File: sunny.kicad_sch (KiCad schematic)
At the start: 53 parts, among them J2 Screw_Terminal_01x03, Q1 FQPF7N90C, T1 7508112339, U10 Optocoupler_DC_PhotoNPN_AKEC, U11 TL431D, U4 MIC4684, U5 UC3842N, U9 AP2112K-3.3, X2 B2P-VH

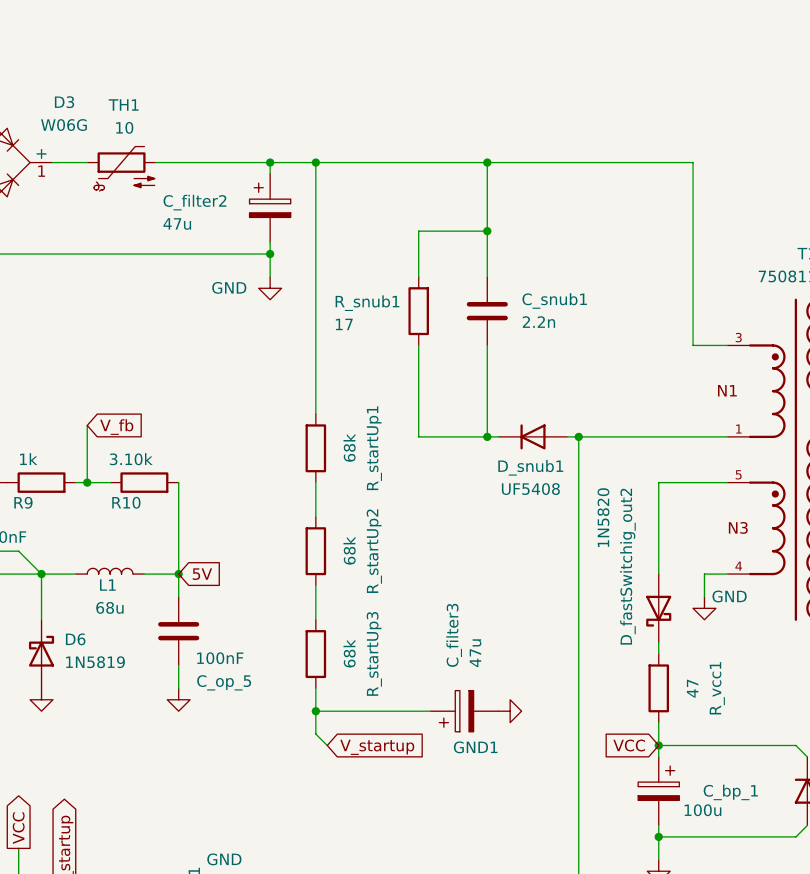
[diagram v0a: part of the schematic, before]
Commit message: Initialtes
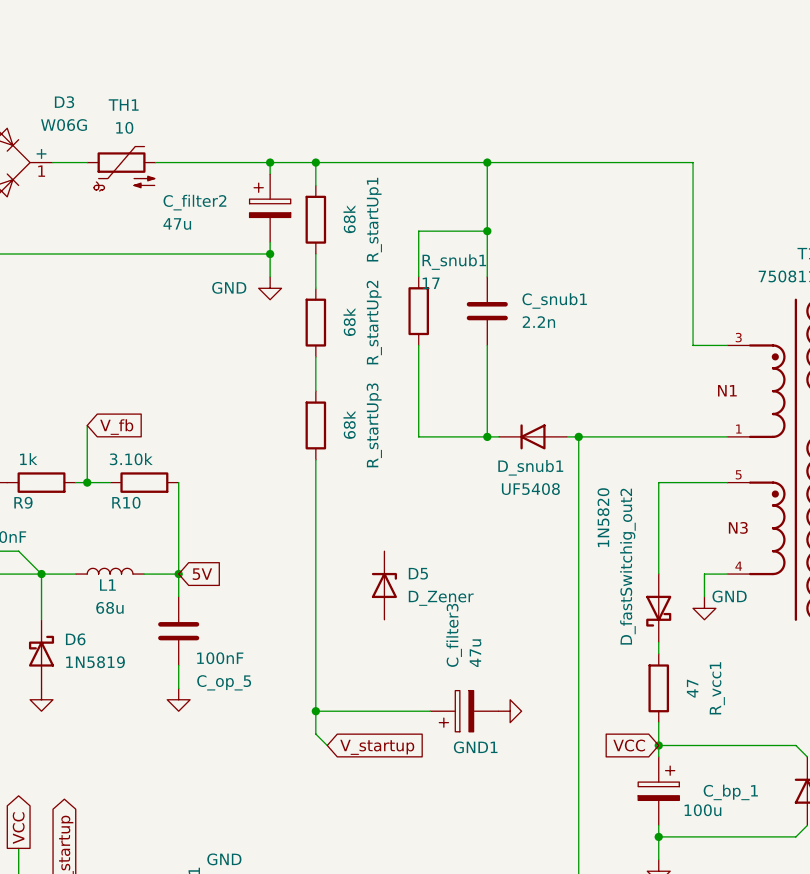
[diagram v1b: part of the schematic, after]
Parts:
- added D5: D_Zener, Diode_THT:D_5KP_P12.70mm_Horizontal, symbol Device:D_Zener
- U5: footprint UC3842N:DIP794W45P254L959H508Q8 -> kaam25_footprints_symbol:DIP794W45P254L959H508Q8
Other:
- moved on the sheet: R_startUp1, R_startUp2, R_startUp3
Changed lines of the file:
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@@
 	)
 	(junction
-		(at 148.59 38.1)
+		(at 186.69 102.87)
 		(diameter 0)
 		(color 0 0 0 0)
 	)
 	(junction
-		(at 186.69 102.87)
+		(at 76.2 81.28)
 		(diameter 0)
 		(color 0 0 0 0)
 	)
 	(junction
-		(at 76.2 81.28)
+		(at 148.59 99.06)
 		(diameter 0)
 		(color 0 0 0 0)
@@
 	)
 	(junction
-		(at 148.59 99.06)
+		(at 148.59 38.1)
 		(diameter 0)
 		(color 0 0 0 0)
@@
 	(wire
 		(pts
-			(xy 148.59 96.52) (xy 148.59 99.06)
+			(xy 148.59 71.12) (xy 148.59 99.06)
 		)
 		(stroke
@@
 	(wire
 		(pts
-			(xy 148.59 85.09) (xy 148.59 88.9)
+			(xy 148.59 59.69) (xy 148.59 63.5)
 		)
 		(stroke
@@
 	(wire
 		(pts
-			(xy 148.59 38.1) (xy 148.59 66.04)
+			(xy 148.59 38.1) (xy 148.59 40.64)
 		)
 		(stroke
@@
 	(wire
 		(pts
-			(xy 148.59 73.66) (xy 148.59 77.47)
+			(xy 148.59 48.26) (xy 148.59 52.07)
 		)
 		(stroke
@@
 			)
 		)
-		(property "Footprint" "UC3842N:DIP794W45P254L959H508Q8"
+		(property "Footprint" "kaam25_footprints_symbol:DIP794W45P254L959H508Q8"
 			(at 97.79 137.16 0)
 			(hide yes)
@@
 		(dnp no)
 		(property "Reference" "R_snub1"
-			(at 150.622 53.594 0)
+			(at 160.274 49.022 0)
 			(show_name no)
 			(do_not_autoplace no)
@@
 		)
 		(property "Value" "17"
-			(at 150.622 56.134 0)
+			(at 160.274 51.562 0)
 			(show_name no)
 			(do_not_autoplace no)
@@
 	(symbol
 		(lib_id "Device:R")
-		(at 148.59 92.71 0)
+		(at 148.59 67.31 0)
 		(mirror x)
 		(unit 1)
@@
 		(dnp no)
 		(property "Reference" "R_startUp3"
-			(at 154.94 92.71 90)
+			(at 154.94 67.31 90)
 			(show_name no)
 			(do_not_autoplace no)
@@
 		)
 		(property "Value" "68k"
-			(at 152.4 92.71 90)
+			(at 152.4 67.31 90)
 			(show_name no)
 			(do_not_autoplace no)
@@
 		)
 		(property "Footprint" "Resistor_THT:R_Axial_DIN0309_L9.0mm_D3.2mm_P20.32mm_Horizontal"
-			(at 146.812 92.71 90)
+			(at 146.812 67.31 90)
 			(hide yes)
 			(show_name no)
@@
 		)
 		(property "Datasheet" ""
-			(at 148.59 92.71 0)
+			(at 148.59 67.31 0)
 			(hide yes)
 			(show_name no)
@@
 		)
 		(property "Description" "starup voltage flows through before aux winding start supplying it, HV resistor, 0.5W, 310Volts"
-			(at 148.59 92.71 0)
+			(at 148.59 67.31 0)
 			(hide yes)
 			(show_name no)
@@
 	(symbol
 		(lib_id "Device:R")
-		(at 148.59 81.28 0)
+		(at 148.59 55.88 0)
 		(mirror x)
 		(unit 1)
@@
 		(dnp no)
 		(property "Reference" "R_startUp2"
-			(at 154.94 81.28 90)
+			(at 154.94 55.88 90)
 			(show_name no)
 			(do_not_autoplace no)
@@
 		)
 		(property "Value" "68k"
-			(at 152.4 81.28 90)
+			(at 152.4 55.88 90)
 			(show_name no)
 			(do_not_autoplace no)
@@
 		)
 		(property "Footprint" "Resistor_THT:R_Axial_DIN0309_L9.0mm_D3.2mm_P20.32mm_Horizontal"
-			(at 146.812 81.28 90)
+			(at 146.812 55.88 90)
 			(hide yes)
 			(show_name no)
@@
 		)
 		(property "Datasheet" ""
-			(at 148.59 81.28 0)
+			(at 148.59 55.88 0)
 			(hide yes)
 			(show_name no)
@@
 		)
 		(property "Description" "starup voltage flows through before aux winding start supplying it, HV resistor,0.5W, 310V"
-			(at 148.59 81.28 0)
+			(at 148.59 55.88 0)
 			(hide yes)
 			(show_name no)
@@
 	(symbol
 		(lib_id "Device:R")
-		(at 148.59 69.85 0)
+		(at 148.59 44.45 0)
 		(mirror x)
 		(unit 1)
@@
 		(dnp no)
 		(property "Reference" "R_startUp1"
-			(at 154.94 69.85 90)
+			(at 154.94 44.45 90)
 			(show_name no)
 			(do_not_autoplace no)
@@
 		)
 		(property "Value" "68k"
-			(at 152.4 69.85 90)
+			(at 152.4 44.45 90)
 			(show_name no)
 			(do_not_autoplace no)
@@
 		)
 		(property "Footprint" "Resistor_THT:R_Axial_DIN0309_L9.0mm_D3.2mm_P20.32mm_Horizontal"
-			(at 146.812 69.85 90)
+			(at 146.812 44.45 90)
 			(hide yes)
 			(show_name no)
@@
 		)
 		(property "Datasheet" ""
-			(at 148.59 69.85 0)
+			(at 148.59 44.45 0)
 			(hide yes)
 			(show_name no)
@@
 		)
 		(property "Description" "starup voltage flows through before aux winding start supplying it, HV resistor,0.5W, 310V"
-			(at 148.59 69.85 0)
+			(at 148.59 44.45 0)
 			(hide yes)
 			(show_name no)
@@
 					(unit 1)
 				)
+			)
+		)
+	)
+	(symbol
+		(lib_id "Device:D_Zener")
+		(at 156.21 85.09 270)
+		(unit 1)
+		(body_style 1)
+		(exclude_from_sim no)
+		(in_bom yes)
+		(on_board yes)
+		(in_pos_files yes)
+		(dnp no)
+		(fields_autoplaced yes)
+		(property "Reference" "D5"
+			(at 158.75 83.8199 90)
+			(show_name no)
+			(do_not_autoplace no)
+			(effects
+				(font
+					(size 1.27 1.27)
+				)
+				(justify left)
+			)
+		)
+		(property "Value" "D_Zener"
+			(at 158.75 86.3599 90)
+			(show_name no)
+			(do_not_autoplace no)
+			(effects
+				(font
+					(size 1.27 1.27)
+				)
+				(justify left)
+			)
+		)
+		(property "Footprint" "Diode_THT:D_5KP_P12.70mm_Horizontal"
+			(at 156.21 85.09 0)
+			(hide yes)
+			(show_name no)
+			(do_not_autoplace no)
+			(effects
+				(font
+					(size 1.27 1.27)
+				)
+			)
+		)
+		(property "Datasheet" ""
+			(at 156.21 85.09 0)
+			(hide yes)
+			(show_name no)
+			(do_not_autoplace no)
+			(effects
+				(font
+					(size 1.27 1.27)
+				)
+			)
+		)
+		(property "Description" "Zener diode"
+			(at 156.21 85.09 0)
+			(hide yes)
+			(show_name no)
+			(do_not_autoplace no)
+			(effects
+				(font
+					(size 1.27 1.27)
+				)
+			)
+		)
+		(pin "1"
+		)
+		(pin "2"
+		)
+		(instances
+			(project "chandra_queenofnight"
+				(path "/fe3f1796-d4c1-46ec-bdb5-a29f35c8d4af/43d0d107-b03e-4228-bd2c-42b72694ee16"
+					(reference "D5")
+					(unit 1)
+				)

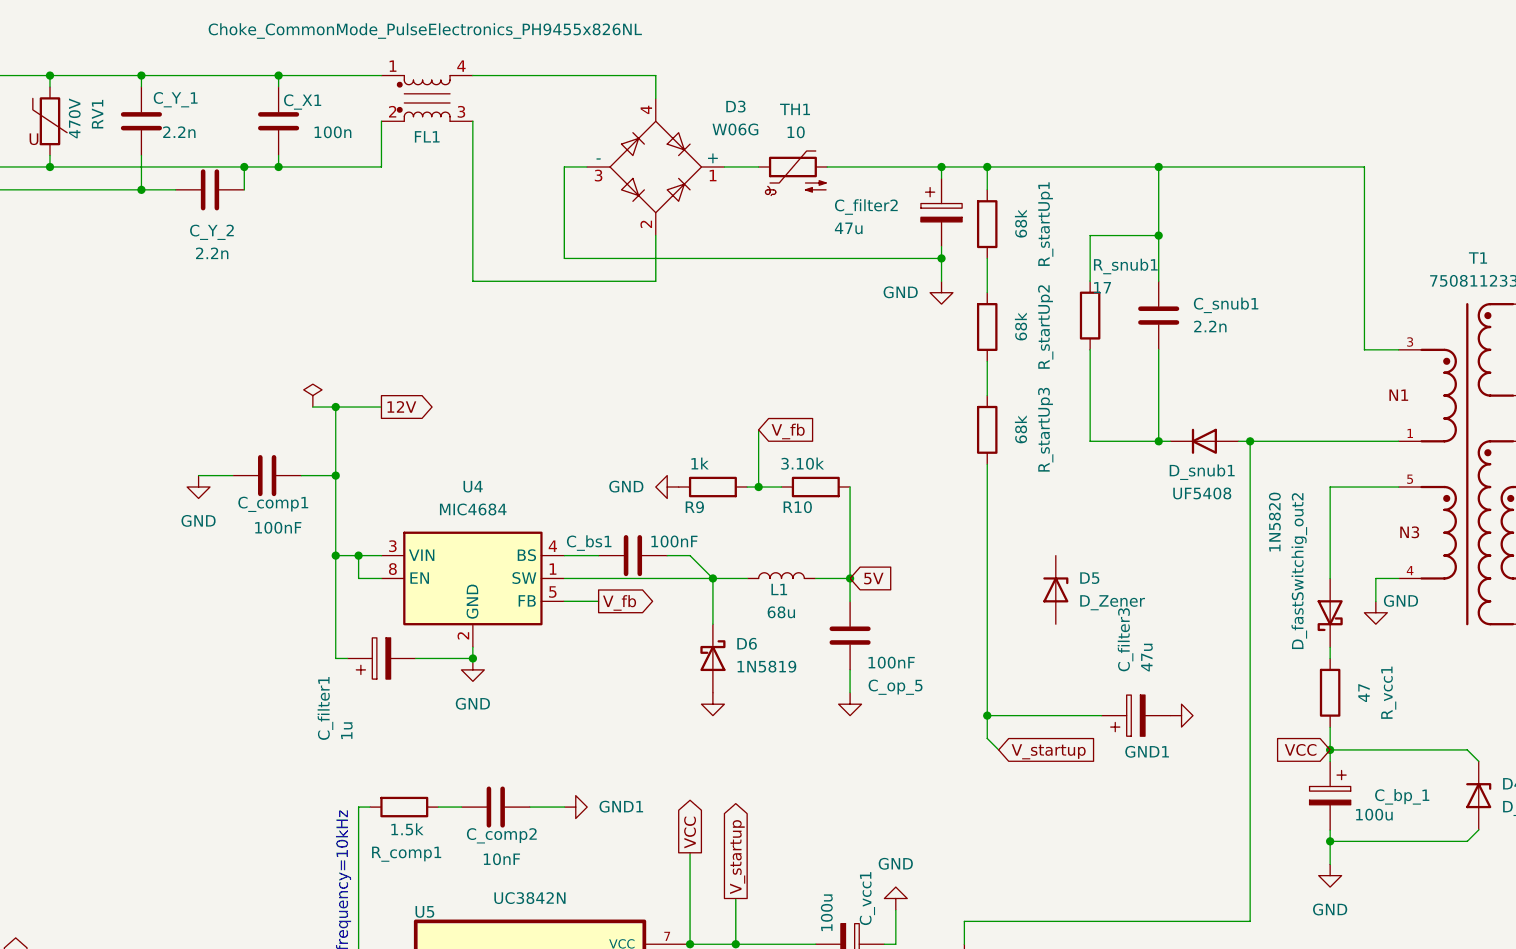
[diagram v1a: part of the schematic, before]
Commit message: Initialtes 130426
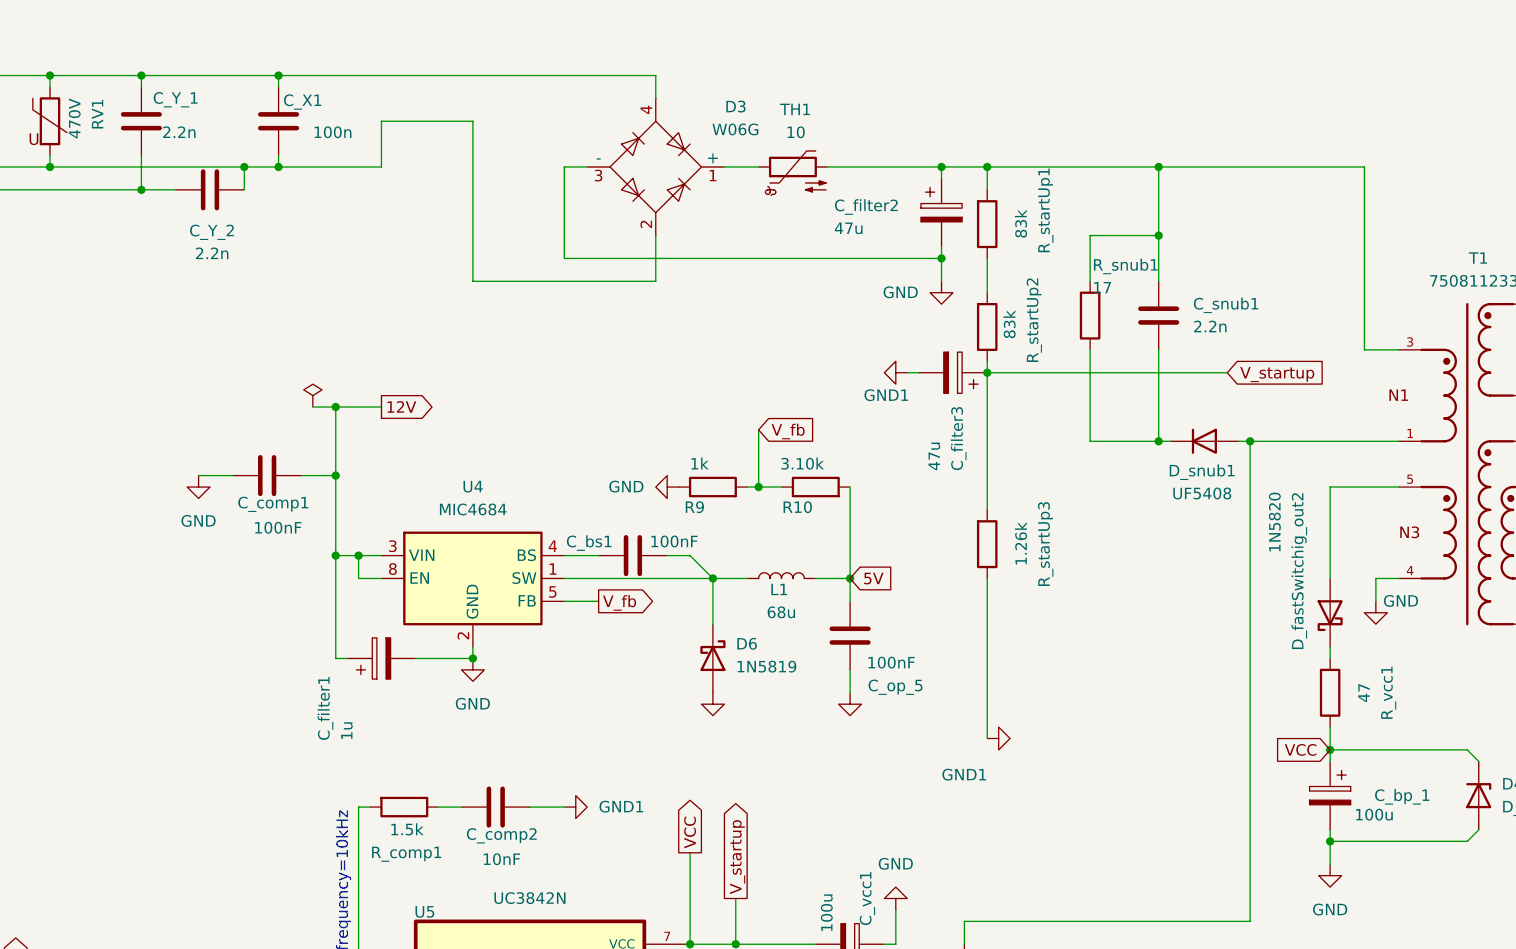
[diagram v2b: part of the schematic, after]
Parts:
- removed D5: D_Zener, Diode_THT:D_5KP_P12.70mm_Horizontal, symbol Device:D_Zener
- removed FL1: Choke_CommonMode_PulseElectronics_PH9455x826NL, Inductor_THT:L_CommonMode_PulseElectronics_PH9455xxx6NL_2, symbol Filter:Choke_CommonMode_PulseElectronics_PH9455x826NL
- R_startUp1, R_startUp2: value 68k -> 83k
- R_startUp3: value 68k -> 1.26k
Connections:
- net GND1: now also R_startUp3.1
- net L: now also D3.4
- net N: now also D3.2
- net VCC: now also R_startUp2.1, R_startUp3.2; no longer R_startUp3.1
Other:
- moved on the sheet: C_filter3, R_startUp3
